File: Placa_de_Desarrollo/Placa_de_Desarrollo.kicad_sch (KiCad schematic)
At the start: 43 parts, among them J1 SD_Card, J10 5V, J11 3.3V, J12 ADC_VREF, J13 GND, J14 AGND, J15 VSYS, J16 3V3_EN, J2 DEVICE I2C1, J3 DEVICE I2C0, J4 Conn_01x01, J5 Conn_01x01, J6 Conn_01x01, J7 Conn_01x01, J8 Conn_01x01, J9 Conn_01x01, U1 Pico, U2 LCD-016N002L

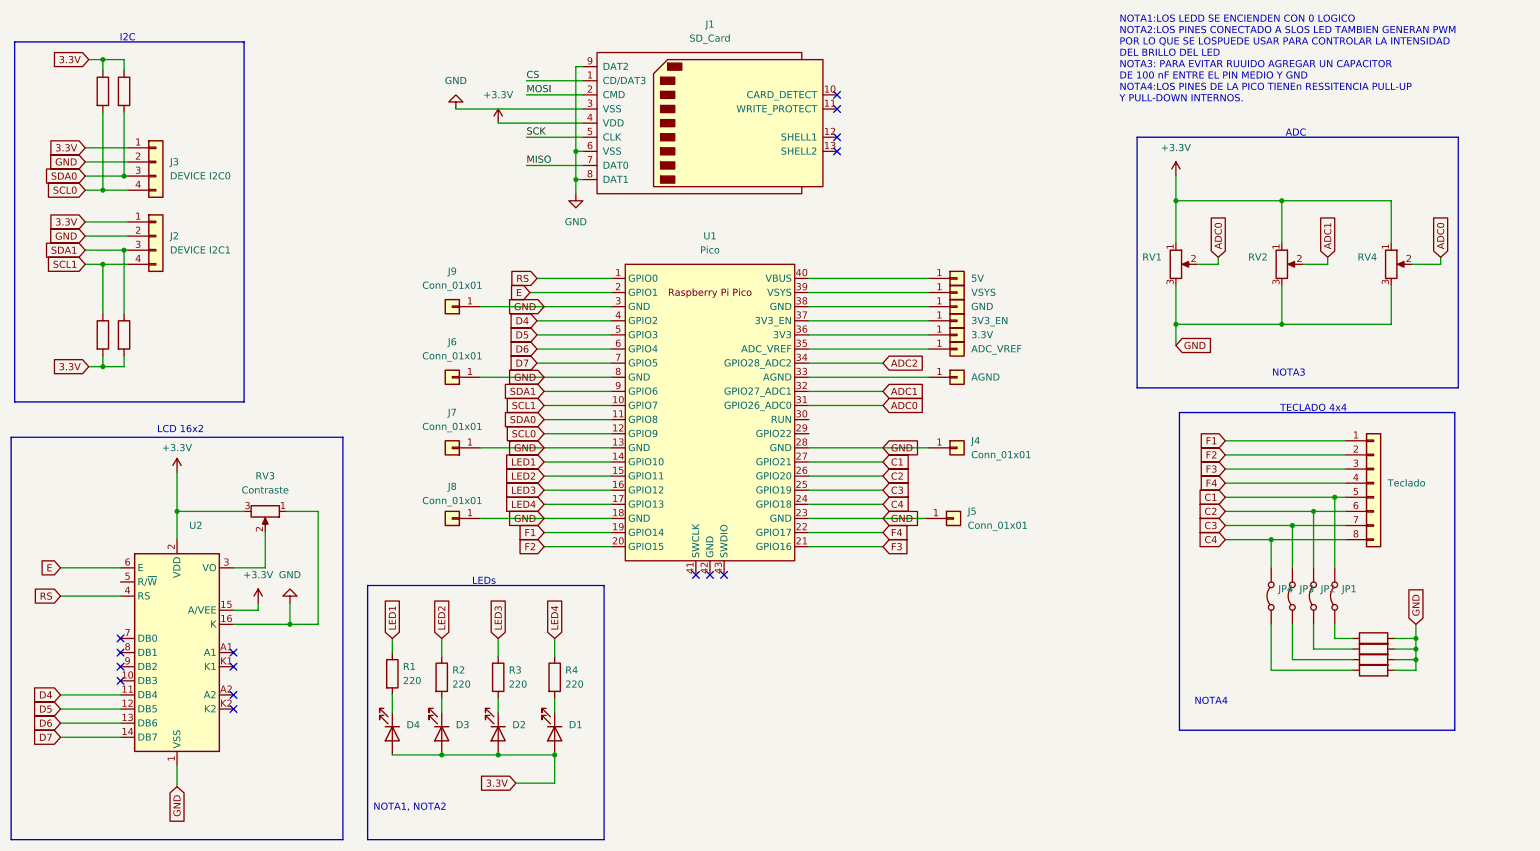
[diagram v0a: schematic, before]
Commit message: Adicion de proyectos anteriores
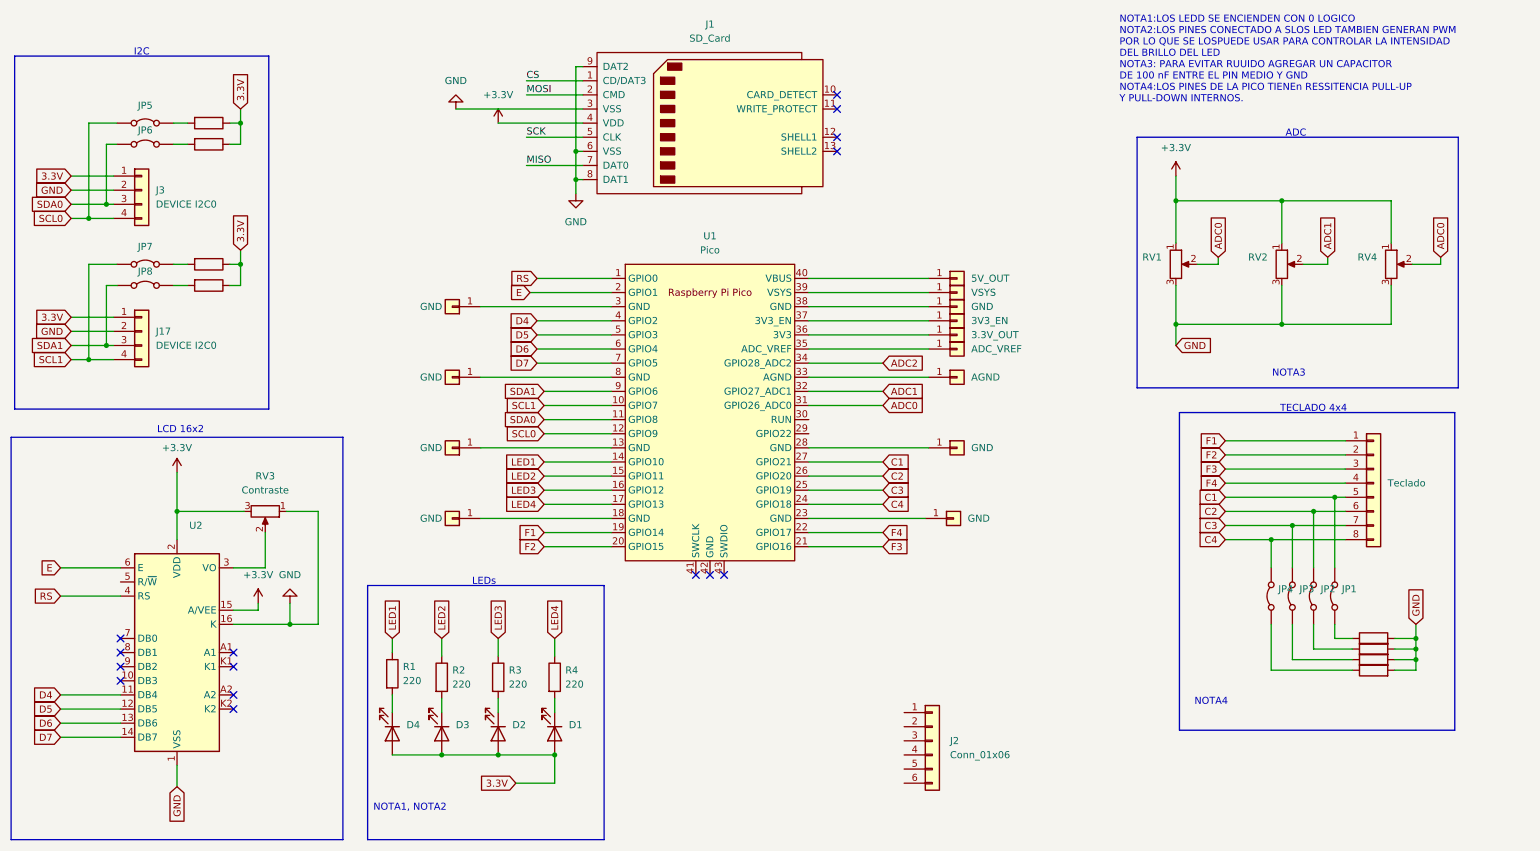
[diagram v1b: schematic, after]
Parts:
- removed J2: DEVICE I2C1, symbol Connector_Generic:Conn_01x04
- removed R11, R12: 4,7k, symbol Device:R
- added J17: DEVICE I2C0, symbol Connector_Generic:Conn_01x04
- added J2: Conn_01x06, symbol Connector_Generic:Conn_01x06
- added JP5, JP6, JP7, JP8: Jumper_2_Bridged, symbol Jumper:Jumper_2_Bridged
- added R13, R14: 4,7k, symbol Device:R
- J10: value 5V -> 5V_OUT
- J11: value 3.3V -> 3.3V_OUT
- J4, J5, J6, J7, J8, J9: value Conn_01x01 -> GND
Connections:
- net 3.3V: now also J17.1 (Pin_1), R13.1, R14.1
- net GND: now also J17.2 (Pin_2); no longer J4.1 (Pin_1), J5.1 (Pin_1), J6.1 (Pin_1), J7.1 (Pin_1), J8.1 (Pin_1), J9.1 (Pin_1), U1.13 (GND), U1.18 (GND), U1.23 (GND), U1.28 (GND), U1.3 (GND), U1.8 (GND)
- net SCL0: now also JP5.1 (A); no longer R9.2
- net SCL1: now also J17.4 (Pin_4), JP7.1 (A)
- net SDA0: now also JP6.1 (A); no longer R10.2
- net SDA1: now also J17.3 (Pin_3), JP8.1 (A)
- new net: J7.1 (Pin_1), U1.13 (GND)
- new net: JP5.2 (B), R9.2
- new net: J5.1 (Pin_1), U1.23 (GND)
- new net: J8.1 (Pin_1), U1.18 (GND)
- new net: J4.1 (Pin_1), U1.28 (GND)
- new net: J9.1 (Pin_1), U1.3 (GND)
- new net: J6.1 (Pin_1), U1.8 (GND)
- new net: JP6.2 (B), R10.2
- new net: JP8.2 (B), R14.2
- new net: JP7.2 (B), R13.2
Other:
- moved on the sheet: J3
